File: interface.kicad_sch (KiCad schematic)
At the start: 31 parts, among them J5 5034801200, SW1 TS35CA, U10 LIS3DH, U11 AP3602AKTR-G1, U8 DRV2603RUNT, U9 TPS61040DBV

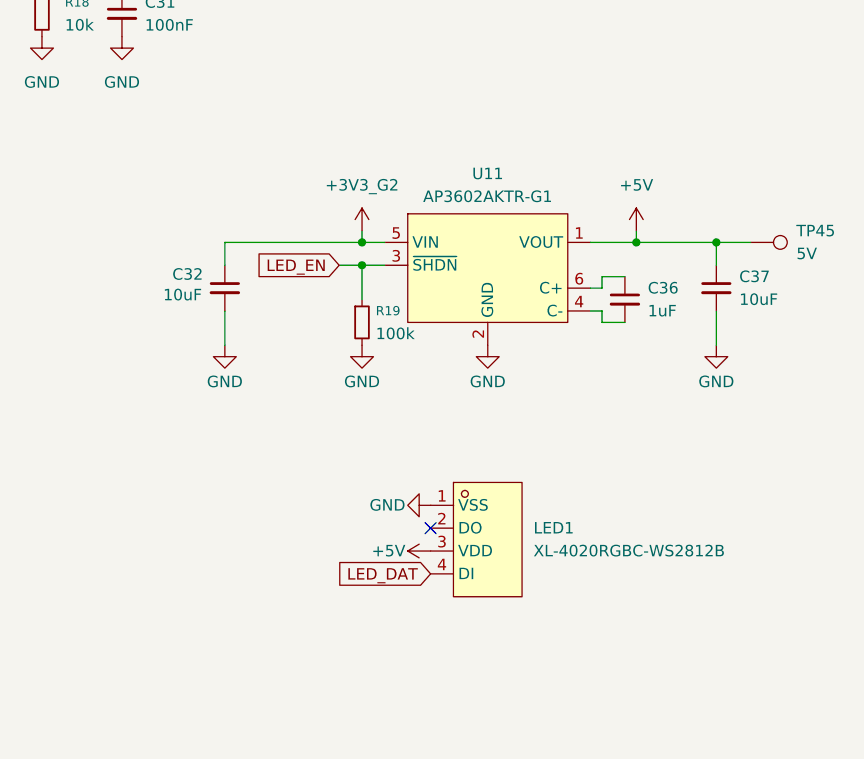
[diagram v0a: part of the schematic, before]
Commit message: progress before minor redesign
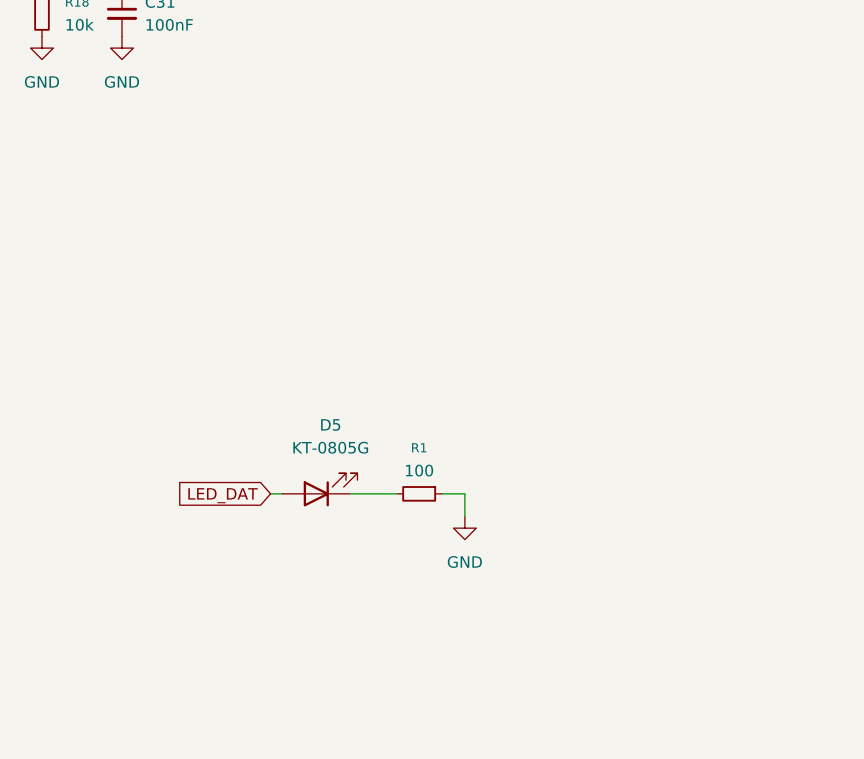
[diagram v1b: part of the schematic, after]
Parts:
- removed C32, C37: 10uF, Capacitor_SMD:C_0402_1005Metric, symbol Device:C_Small
- removed C36: 1uF, Capacitor_SMD:C_0402_1005Metric, symbol Device:C_Small
- removed LED1: XL-4020RGBC-WS2812B, XL-4020RGBC-2812B:LED-SMD_4P-L4.0-W1.7_XL-4020RGBC-WS2812B, symbol XL-4020RGBC-2812B:XL-4020RGBC-WS2812B
- removed R19: 100k, Resistor_SMD:R_0402_1005Metric, symbol Device:R_Small
- removed TP45: 5V, TestPoint:TestPoint_Pad_D1.0mm, symbol Connector:TestPoint
- removed U11: AP3602AKTR-G1, AP3602AKTR-G1:SOT-23-6_L2.9-W1.6-P0.95-LS2.8-BR, symbol AP3602AKTR-G1:AP3602AKTR-G1
- added D5: KT-0805G, Diode_SMD:D_0805_2012Metric, symbol Device:LED
- added R1: 100, Resistor_SMD:R_0402_1005Metric, symbol Device:R_Small
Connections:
- net GND: now also R1.1
- net LED_DAT: now also D5.2 (A)
- new net: D5.1 (K), R1.2
- no-connect marks 8 -> 7
